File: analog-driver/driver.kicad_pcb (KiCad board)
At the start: 2 copper layers, 81 x 23.4 mm, 18 parts, among them J1 Conn_01x02, J2 Barrel_Jack, J3 Barrel_Jack, M1 Fan_4pin, U1 AL8805W5-7, U2 LM2941S

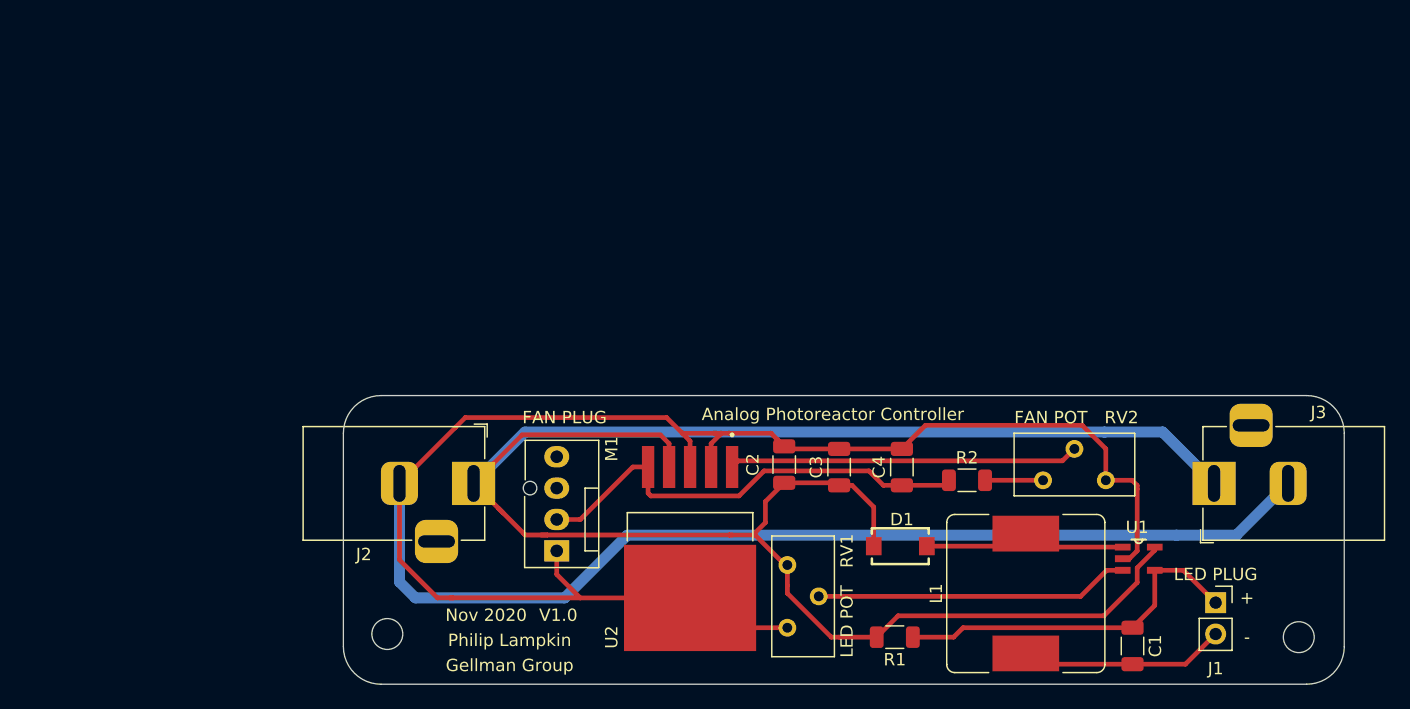
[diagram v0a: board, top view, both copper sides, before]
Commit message: analog driver 1.0.0
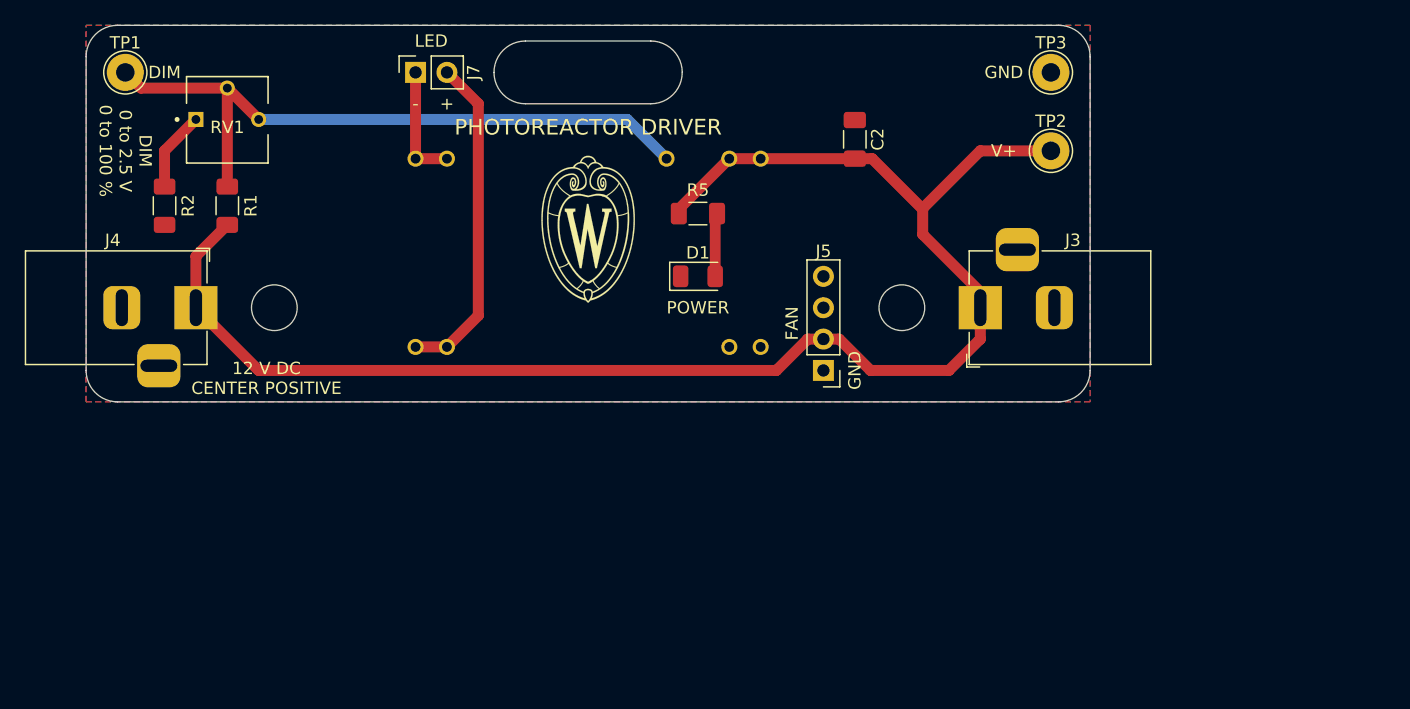
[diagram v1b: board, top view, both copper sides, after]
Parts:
- removed C1: 1uF, Capacitor_SMD:C_1206_3216Metric
- removed C3: 0.47uF, Capacitor_SMD:C_1206_3216Metric
- removed C4: 22uF, Capacitor_SMD:C_1206_3216Metric
- removed J1: Conn_01x02, Connector_PinSocket_2.54mm:PinSocket_1x02_P2.54mm_Vertical
- removed J2: Barrel_Jack, Connector_BarrelJack:BarrelJack_Horizontal
- removed L1: 33uH, Inductor_SMD:L_Bourns_SRR1260
- removed M1: Fan_4pin, Connector:FanPinHeader_1x04_P2.54mm_Vertical
- removed the REF** at (110.7, 128.0)
- removed the REF** at (184.5, 128.3)
- removed RV2: 5kOhm1, Potentiometer_THT:Potentiometer_Bourns_3296Y_Vertical
- removed U1: AL8805W5-7, AL8805W5-7:SOT95P280X130-5N
- added G***: LOGO, footprints:logo, F.Cu at (127.0, 95.2)
- added J4: Barrel_Jack, Connector_BarrelJack:BarrelJack_Horizontal, F.Cu at (95.2, 101.6)
- added J5: Conn_01x04, Connector_PinHeader_2.54mm:PinHeader_1x04_P2.54mm_Vertical, F.Cu at (146.1, 106.7)
- added J7: Conn_01x02, Connector_PinSocket_2.54mm:PinSocket_1x02_P2.54mm_Vertical, F.Cu at (113.0, 82.5)
- added R5: 1k, Resistor_SMD:R_1206_3216Metric_Pad1.30x1.75mm_HandSolder, F.Cu at (135.9, 94.0)
- added REF**: MountingHole_3.7mm, MountingHole:MountingHole_3.7mm, F.Cu at (152.4, 101.6)
- added REF**: MountingHole_3.7mm, MountingHole:MountingHole_3.7mm, F.Cu at (101.6, 101.6)
- added TP1: TestPoint, TestPoint:TestPoint_THTPad_D3.0mm_Drill1.5mm, F.Cu at (89.5, 82.5)
- added TP2: TestPoint, TestPoint:TestPoint_THTPad_D3.0mm_Drill1.5mm, F.Cu at (164.5, 88.9)
- added TP3: TestPoint, TestPoint:TestPoint_THTPad_D3.0mm_Drill1.5mm, F.Cu at (164.5, 82.5)
- C2: value 2.2uF -> 10u; footprint Capacitor_SMD:C_1206_3216Metric -> Capacitor_SMD:C_1206_3216Metric_Pad1.33x1.80mm_HandSolder
- D1: value MBRA140 -> LED; footprint MBRA140:SMA-DIODE -> LED_SMD:LED_1206_3216Metric
- R1: value 0.3R -> 10k; footprint Resistor_SMD:R_1206_3216Metric -> Resistor_SMD:R_1206_3216Metric_Pad1.30x1.75mm_HandSolder
- R2: value 8KOhm -> 470; footprint Resistor_SMD:R_1206_3216Metric -> Resistor_SMD:R_1206_3216Metric_Pad1.30x1.75mm_HandSolder
- RV1: value 100KOhm -> 2.2k; footprint Potentiometer_THT:Potentiometer_Bourns_3296Y_Vertical -> footprints:TRIM_3362P-1-202TLF
- U2: value LM2941S -> LDD-1500L; footprint LM2941S:VREG_TPS79625KTTR -> LDD-1500L:LDD1500L; moved to B.Cu
- moved R2 68.7 mm to (92.7, 93.3), turned to 270 degrees
- moved R1 64.3 mm to (97.8, 93.3), turned to 90 degrees
- moved RV1 57.9 mm to (97.8, 86.4), turned to 0 degrees
- moved D1 27.3 mm to (135.9, 99.1), turned to 0 degrees
- moved C2 26.9 mm to (148.6, 88.0)
- moved J3 23.7 mm to (158.8, 101.6)
- moved U2 21.1 mm to (141.0, 104.8), turned to 90 degrees
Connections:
- R1 pad 1: Net-(C1-Pad1) -> +12V
- R1 pad 2: +12V -> Net-(R1-Pad2)
- R2 pad 1: Net-(C4-Pad1) -> Net-(R2-Pad1)
- R2 pad 2: Net-(R2-Pad2) -> GND
- RV1 pad 1: +12V -> Net-(R2-Pad1)
- RV1 pad 2: Net-(RV1-Pad2) -> Net-(R1-Pad2)
- RV1 pad 3: GND -> Net-(R1-Pad2)
- U2 pad 1: Net-(RV2-Pad2) -> GND
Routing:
- net GND: track 217.1 -> 0.00 mm
- net Net-(R1-Pad2): track 0.00 -> 54.7 mm
- net +12V: track 168.8 -> 126.1 mm
- net Net-(C4-Pad1): track 38.4 -> 0.00 mm
- net Net-(C1-Pad1): track 29.5 -> 0.00 mm
- net Net-(RV2-Pad2): track 28.3 -> 0.00 mm
- net Net-(J7-Pad2): track 0.00 -> 26.9 mm
- net Net-(RV1-Pad2): track 25.5 -> 0.00 mm
- net Net-(C1-Pad2): track 16.7 -> 0.00 mm
- net Net-(D1-PadA): track 16.7 -> 0.00 mm
- net Net-(J7-Pad1): track 0.00 -> 9.52 mm
- net Net-(R2-Pad1): track 0.00 -> 6.49 mm
- net Net-(D1-Pad2): track 0.00 -> 5.14 mm
- net Net-(R2-Pad2): track 4.70 -> 0.00 mm
- added copper zone on B.Cu, net GND
- added copper zone on F.Cu, net GND
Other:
- board size 81 x 23.4 mm -> 81.3 x 30.5 mm
- net class Default: clearance 0.2 -> 0.381; trace_width 0.25 -> 0.889
- rule trace_clearance: 0.2 -> 0.381
- board text added: "12 V DC CENTER POSITIVE"
- board text added: "DIM"
- board text added: "DIM 0 to 2.5 V 0 to 100 %"
- board text added: "FAN"
- board text added: "GND"
- board text added: "LED"
- board text added: "PHOTOREACTOR DRIVER"
- board text added: "POWER"
- board text added: "REVISION 1.0.0 JANUARY 2021"
- board text added: "V+"
- board text removed: "Analog Photoreactor Controller"
- board text removed: "FAN PLUG"
- board text removed: "FAN POT"
- board text removed: "Gellman Group"
- board text removed: "LED PLUG"
- board text removed: "LED POT"
- board text removed: "Nov 2020"
- board text removed: "Philip Lampkin"
- board text removed: "V1.0"
